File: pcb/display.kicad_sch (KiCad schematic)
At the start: 4 parts

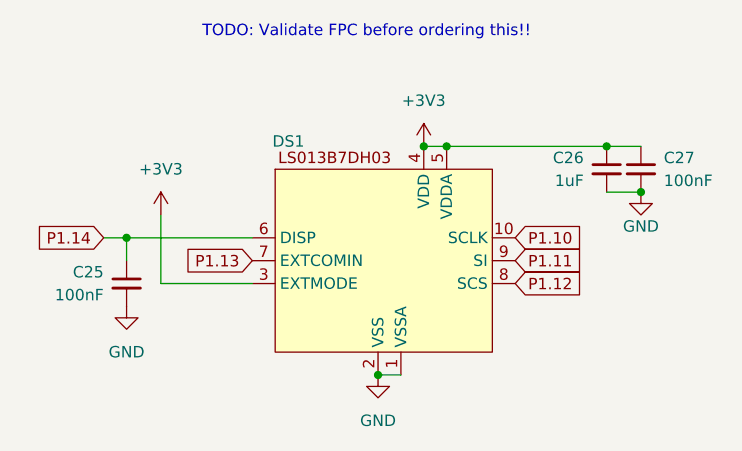
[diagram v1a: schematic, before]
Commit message: mogus
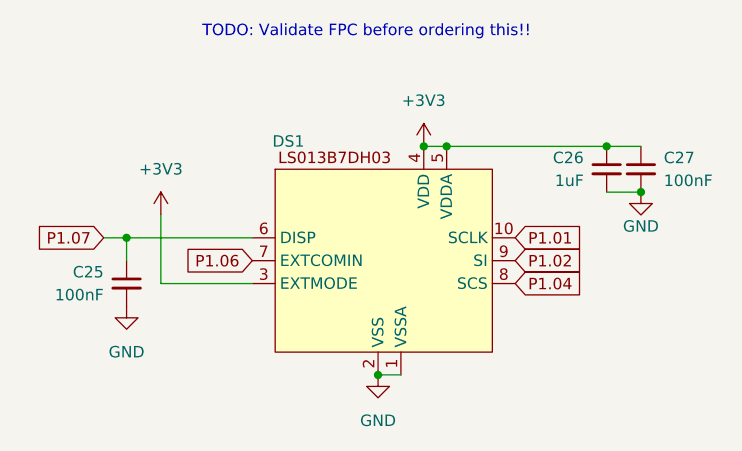
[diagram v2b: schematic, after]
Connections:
- net P1.10 renamed P1.01
- net P1.11 renamed P1.02
- net P1.12 renamed P1.04
- net P1.13 renamed P1.06
- net P1.14 renamed P1.07
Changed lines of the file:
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@@
 		)
 	)
-	(global_label "P1.12"
+	(global_label "P1.07"
 		(shape input)
-		(at 163.83 95.25 0)
+		(at 118.11 90.17 180)
 		(fields_autoplaced yes)
 		(effects
@@
 				(size 1.27 1.27)
 			)
-			(justify left)
+			(justify right)
 		)
 		(property "Intersheetrefs" "${INTERSHEET_REFS}"
-			(at 172.3185 95.25 0)
+			(at 109.6215 90.17 0)
 			(hide yes)
 			(show_name no)
@@
 					(size 1.27 1.27)
 				)
-				(justify left)
+				(justify right)
 			)
 		)
 	)
-	(global_label "P1.11"
+	(global_label "P1.06"
+		(shape input)
+		(at 134.62 92.71 180)
+		(fields_autoplaced yes)
+		(effects
+			(font
+				(size 1.27 1.27)
+			)
+			(justify right)
+		)
+		(property "Intersheetrefs" "${INTERSHEET_REFS}"
+			(at 126.1315 92.71 0)
+			(hide yes)
+			(show_name no)
+			(do_not_autoplace no)
+			(effects
+				(font
+					(size 1.27 1.27)
+				)
+				(justify right)
+			)
+		)
+	)
+	(global_label "P1.02"
 		(shape input)
 		(at 163.83 92.71 0)
@@
 		)
 	)
-	(global_label "P1.14"
-		(shape input)
-		(at 118.11 90.17 180)
-		(fields_autoplaced yes)
-		(effects
-			(font
-				(size 1.27 1.27)
-			)
-			(justify right)
-		)
-		(property "Intersheetrefs" "${INTERSHEET_REFS}"
-			(at 109.6215 90.17 0)
-			(hide yes)
-			(show_name no)
-			(do_not_autoplace no)
-			(effects
-				(font
-					(size 1.27 1.27)
-				)
-				(justify right)
-			)
-		)
-	)
-	(global_label "P1.13"
-		(shape input)
-		(at 134.62 92.71 180)
-		(fields_autoplaced yes)
-		(effects
-			(font
-				(size 1.27 1.27)
-			)
-			(justify right)
-		)
-		(property "Intersheetrefs" "${INTERSHEET_REFS}"
-			(at 126.1315 92.71 0)
-			(hide yes)
-			(show_name no)
-			(do_not_autoplace no)
-			(effects
-				(font
-					(size 1.27 1.27)
-				)
-				(justify right)
-			)
-		)
-	)
-	(global_label "P1.10"
+	(global_label "P1.01"
 		(shape input)
 		(at 163.83 90.17 0)
@@
 			(hide yes)
 			(show_name no)
+			(do_not_autoplace no)
+			(effects
+				(font
+					(size 1.27 1.27)
+				)
+				(justify left)
+			)
+		)
+	)
+	(global_label "P1.04"
+		(shape input)
+		(at 163.83 95.25 0)
+		(fields_autoplaced yes)
+		(effects
+			(font
+				(size 1.27 1.27)
+			)
+			(justify left)
+		)
+		(property "Intersheetrefs" "${INTERSHEET_REFS}"
+			(at 172.3185 95.25 0)
+			(hide yes)
+			(show_name no)
